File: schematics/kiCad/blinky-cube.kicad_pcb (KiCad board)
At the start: 2 copper layers, 86.6 x 49.7 mm, 26 parts, among them J1 Screw_Terminal_01x03, J2 Screw_Terminal_01x03, J3 Screw_Terminal_01x03, SW1 SW_Push, U1 Pico, U2 LM4040LP-3

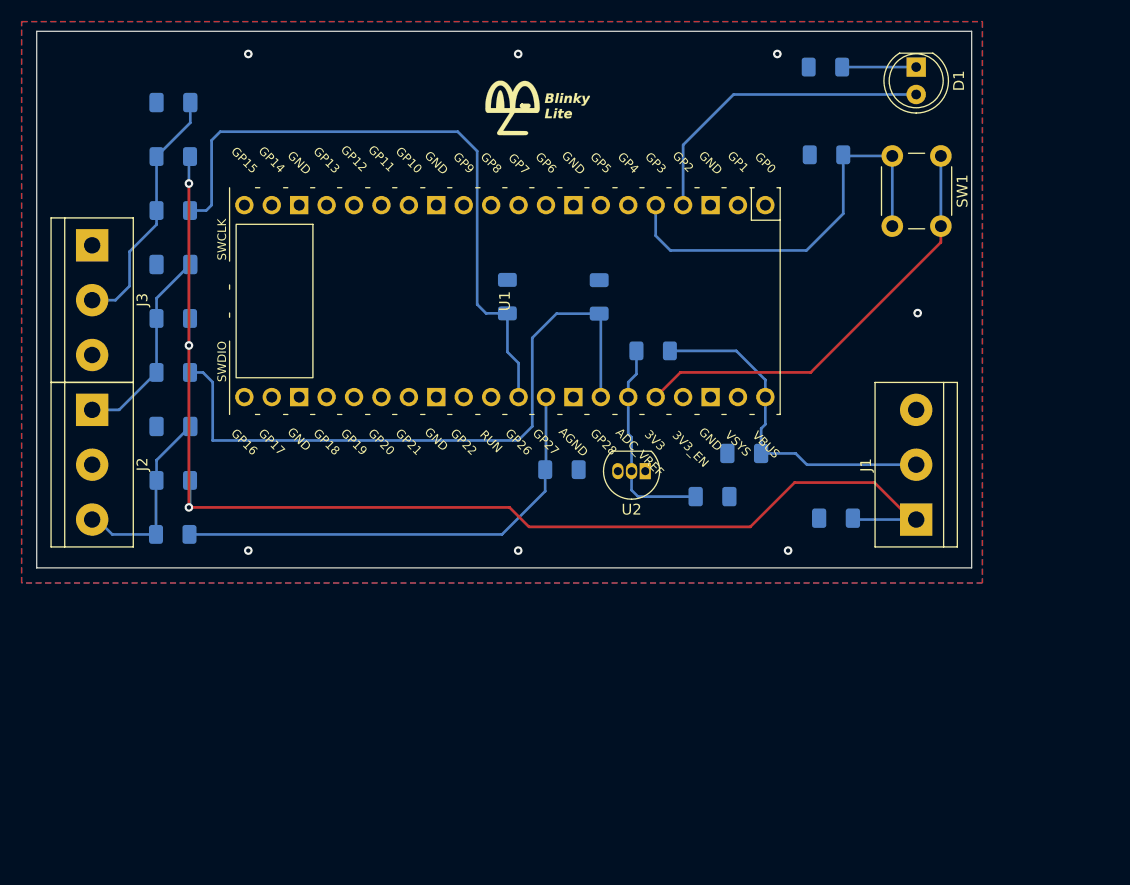
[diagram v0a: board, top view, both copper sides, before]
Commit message: thru hole
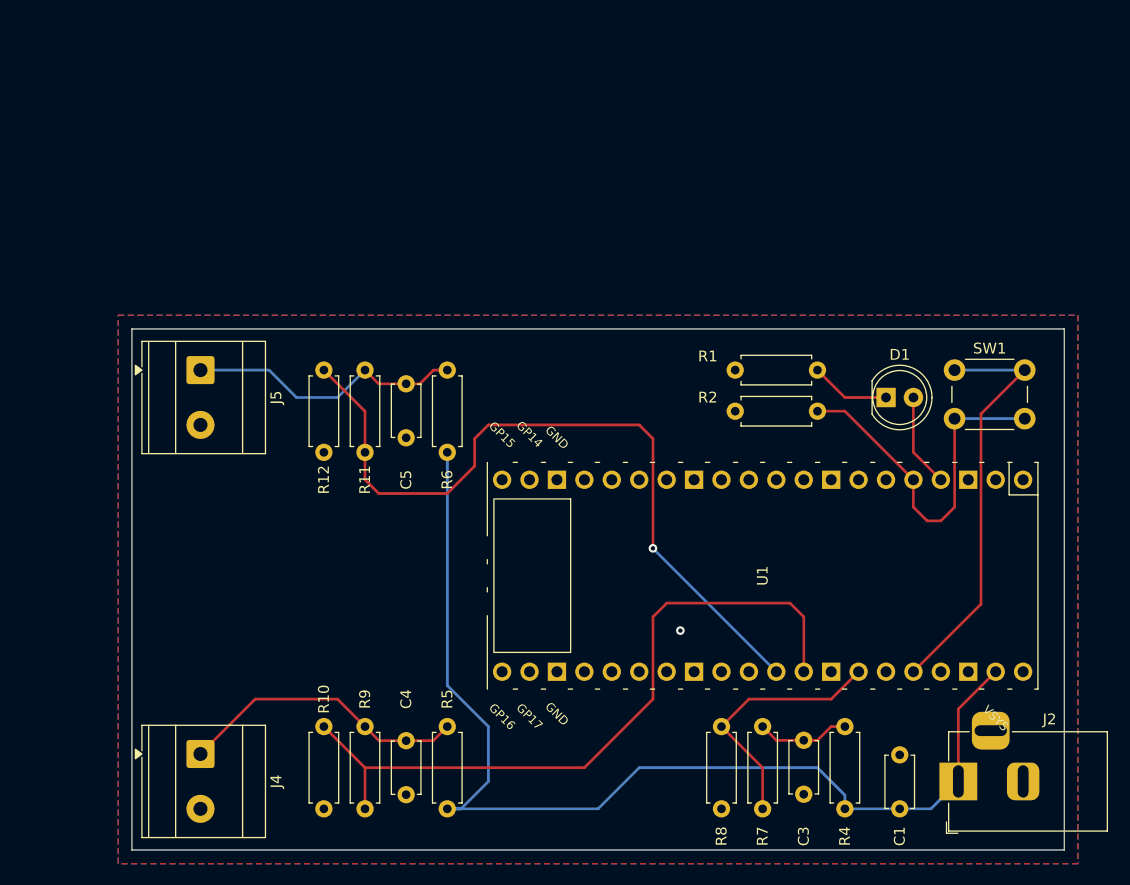
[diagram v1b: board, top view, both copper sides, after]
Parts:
- removed C2, C6: 1uF, Capacitor_SMD:C_1206_3216Metric_Pad1.33x1.80mm_HandSolder
- removed G***: LOGO, blinkyLiteLogo:blinkyLiteLogo
- removed J1, J3: Screw_Terminal_01x03, TerminalBlock:TerminalBlock_bornier-3_P5.08mm
- removed R3: 220, Resistor_SMD:R_1206_3216Metric_Pad1.30x1.75mm_HandSolder
- removed U2: LM4040LP-3, Package_TO_SOT_THT:TO-92_Inline
- added J4: Screw_Terminal_01x02, TerminalBlock_Phoenix:TerminalBlock_Phoenix_MKDS-3-2-5.08_1x02_P5.08mm_Horizontal, F.Cu at (115.6, 116.8)
- added J5: Screw_Terminal_01x02, TerminalBlock_Phoenix:TerminalBlock_Phoenix_MKDS-3-2-5.08_1x02_P5.08mm_Horizontal, F.Cu at (115.6, 81.3)
- C1, C3, C4, C5: footprint Capacitor_SMD:C_1206_3216Metric_Pad1.33x1.80mm_HandSolder -> Capacitor_THT:C_Disc_D4.7mm_W2.5mm_P5.00mm; moved to F.Cu
- J2: value Screw_Terminal_01x03 -> Barrel_Jack_Switch; footprint TerminalBlock:TerminalBlock_bornier-3_P5.08mm -> Connector_BarrelJack:BarrelJack_Horizontal
- R1, R10, R11, R12, R2, R4, R5, R6, R7, R8, R9: footprint Resistor_SMD:R_1206_3216Metric_Pad1.30x1.75mm_HandSolder -> Resistor_THT:R_Axial_DIN0207_L6.3mm_D2.5mm_P7.62mm_Horizontal; moved to F.Cu
- moved J2 87.3 mm to (185.8, 119.4), turned to 180 degrees
- moved C3 73.2 mm to (171.4, 115.6), turned to -90 degrees
- moved R4 72.8 mm to (175.3, 114.3), turned to -90 degrees
- moved R7 63.7 mm to (167.6, 114.3), turned to -90 degrees
- moved R8 41.4 mm to (163.8, 114.3), turned to -90 degrees
- moved C4 36.2 mm to (134.6, 115.6), turned to -90 degrees
- moved C1 35.9 mm to (180.3, 121.9), turned to 90 degrees
- moved U1 34.9 mm to (167.6, 100.3)
- moved R5 34.1 mm to (138.4, 114.3), turned to -90 degrees
- moved C5 33.8 mm to (134.6, 82.5), turned to -90 degrees
- moved R10 32.4 mm to (127.0, 114.3), turned to -90 degrees
- moved R6 32.2 mm to (138.4, 81.3), turned to -90 degrees
- moved D1 30.7 mm to (179.1, 83.8), turned to 0 degrees
- moved R1 29.3 mm to (165.1, 81.3)
- moved R9 25.2 mm to (130.8, 114.3), turned to -90 degrees
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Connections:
- C1 pad 1: Net-(C1-Pad1) -> Net-(U1-VSYS)
- C4 pad 1: Net-(C4-Pad1) -> Net-(J4-Pin_1)
- J2 pad 1: Net-(C3-Pad1) -> Net-(U1-VSYS)
- J2 pad 3: Net-(C4-Pad1) -> unconnected-(J2-Pad3)
- R4 pad 2: Net-(C2-Pad2) -> Net-(U1-VSYS)
- R5 pad 1: Net-(C4-Pad1) -> Net-(J4-Pin_1)
- R5 pad 2: Net-(C2-Pad2) -> Net-(U1-VSYS)
- R6 pad 2: Net-(C2-Pad2) -> Net-(U1-VSYS)
- R9 pad 1: Net-(C4-Pad1) -> Net-(J4-Pin_1)
- U1 pad 35: Net-(R3-Pad2) -> unconnected-(U1-ADC_VREF-Pad35)
- U1 pad 39: unconnected-(U1-Pad39) -> Net-(U1-VSYS)
- U1 pad 40: Net-(C1-Pad1) -> unconnected-(U1-VBUS-Pad40)
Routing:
- net Net-(C2-Pad2): track 114.8 -> 0.00 mm, vias 3 -> 0
- net Net-(U1-VSYS): track 0.00 -> 100.8 mm
- net Net-(U1-GPIO28_ADC2): track 61.1 -> 24.0 mm
- net Net-(C1-Pad1): track 31.7 -> 0.00 mm
- net Net-(J4-Pin_1): track 0.00 -> 27.1 mm
- net Net-(U1-GPIO27_ADC1): track 43.4 -> 66.2 mm
- net Net-(D1-A): track 29.1 -> 8.67 mm
- net Net-(R3-Pad2): track 19.5 -> 0.00 mm
- net Net-(C4-Pad1): track 17.8 -> 0.00 mm
- net Net-(U1-GPIO26_ADC0): track 59.4 -> 69.9 mm, vias 0 -> 1
- net Net-(C3-Pad1): track 18.7 -> 8.67 mm
- net Net-(U1-GPIO3): track 38.7 -> 33.6 mm
- net Net-(J5-Pin_1): track 23.3 -> 26.0 mm
- net Net-(U1-3V3): track 40.4 -> 38.7 mm
- net Net-(D1-K): track 6.86 -> 7.40 mm
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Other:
- board size 86.6 x 49.7 mm -> 86.4 x 48.3 mm
